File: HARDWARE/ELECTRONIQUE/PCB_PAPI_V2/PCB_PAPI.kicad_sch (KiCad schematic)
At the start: 0 parts

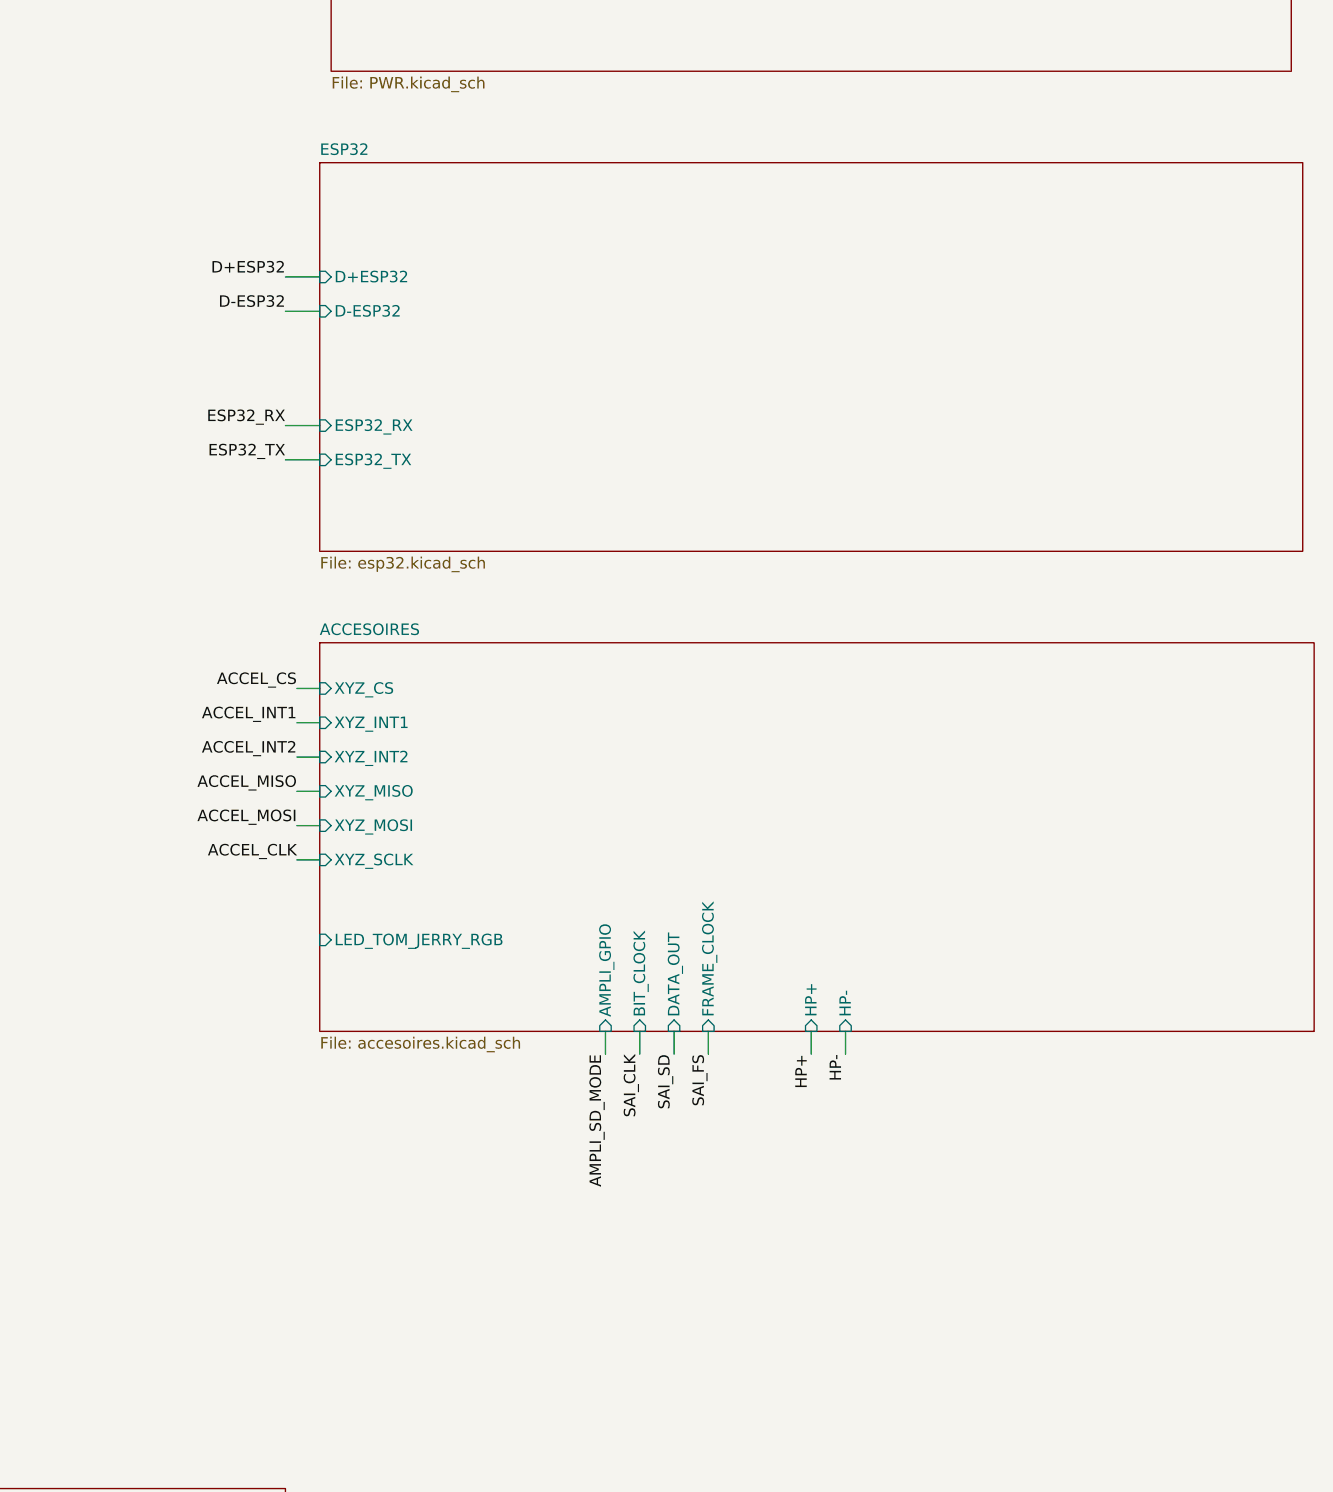
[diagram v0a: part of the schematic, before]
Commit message: up
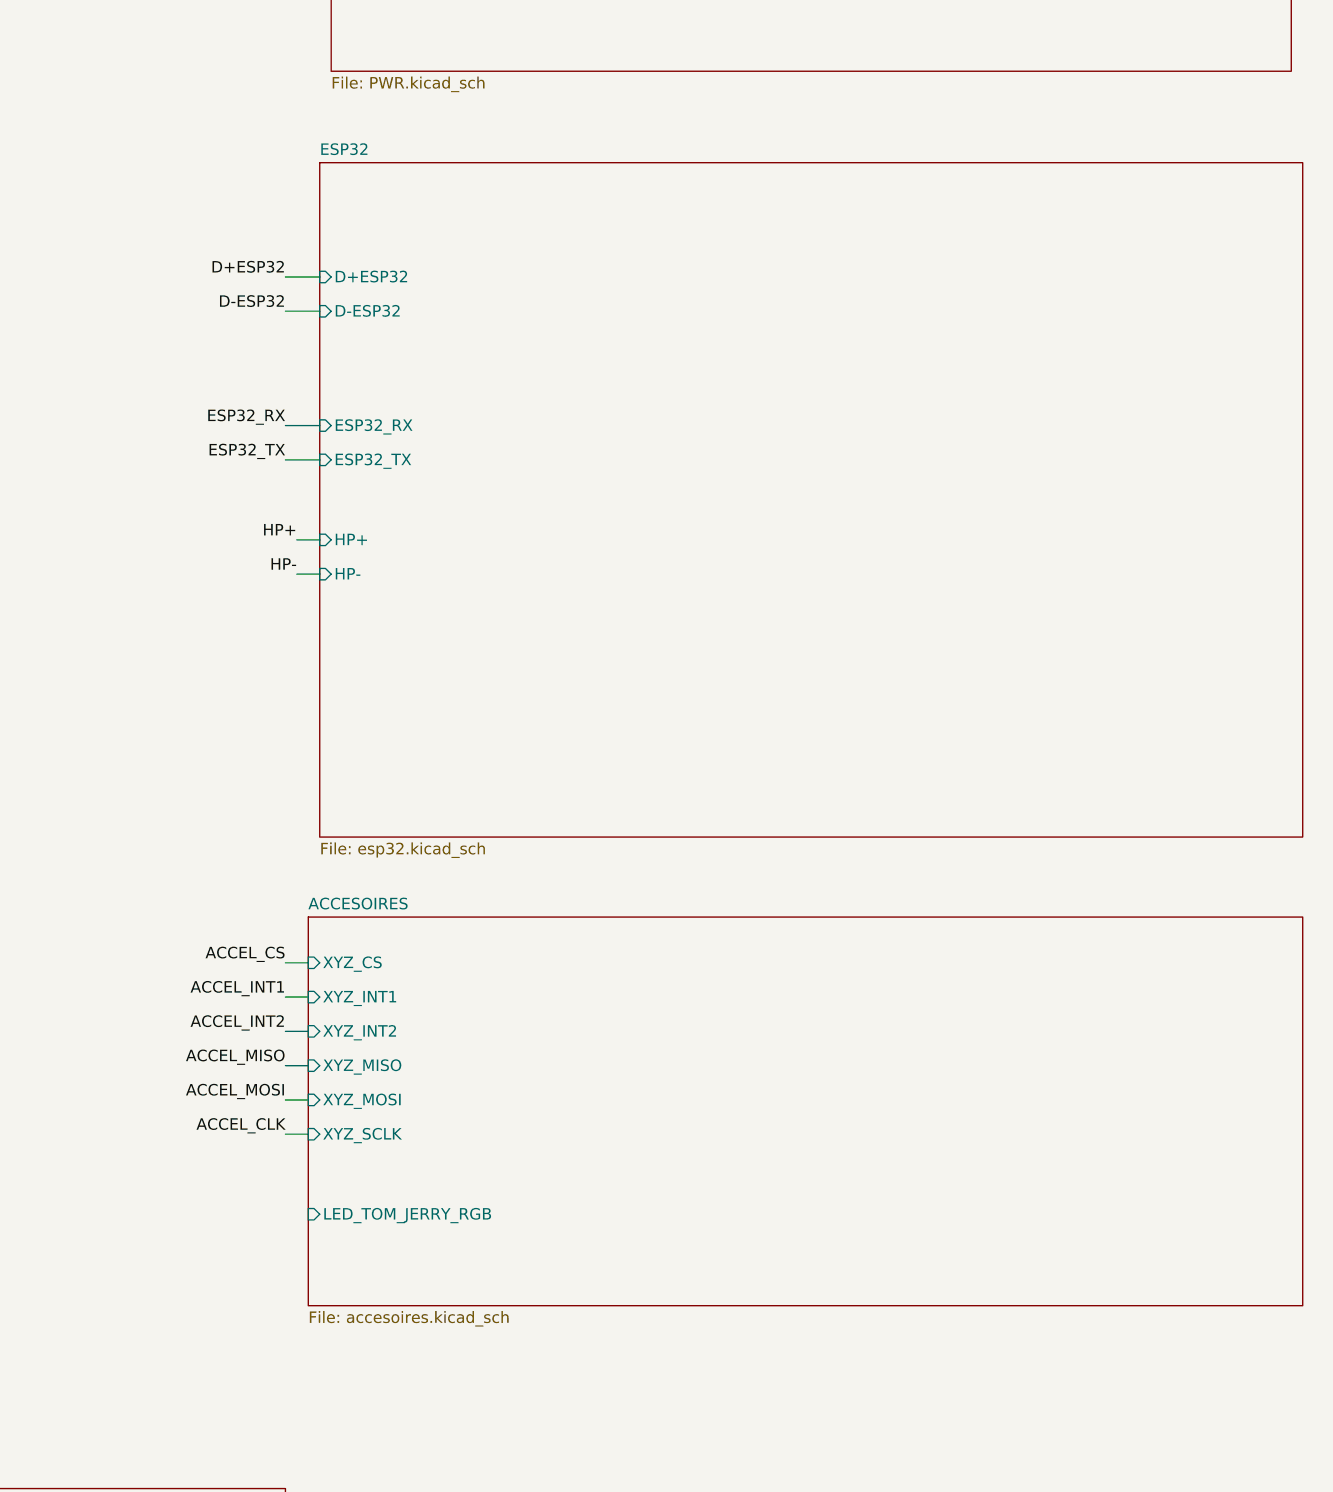
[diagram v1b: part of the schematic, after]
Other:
- sheet ACCESOIRES ports: added none; removed AMPLI_GPIO, BIT_CLOCK, DATA_OUT, FRAME_CLOCK, HP+, HP-
- sheet ESP32 ports: added HP+, HP-; removed none
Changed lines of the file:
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@@
-	(wire
-		(pts
-			(xy 496.57 204.47) (xy 496.57 201.93)
-		)
-		(stroke
-			(width 0)
-			(type default)
-		)
-	)
 	(wire
 		(pts
@@
 	(wire
 		(pts
-			(xy 435.61 167.64) (xy 438.15 167.64)
+			(xy 434.34 198.12) (xy 436.88 198.12)
 		)
 		(stroke
@@
 	(wire
 		(pts
-			(xy 435.61 163.83) (xy 438.15 163.83)
+			(xy 434.34 194.31) (xy 436.88 194.31)
 		)
 		(stroke
@@
 	(wire
 		(pts
-			(xy 435.61 175.26) (xy 438.15 175.26)
+			(xy 434.34 205.74) (xy 436.88 205.74)
 		)
 		(stroke
@@
 	(wire
 		(pts
-			(xy 435.61 179.07) (xy 438.15 179.07)
+			(xy 434.34 209.55) (xy 436.88 209.55)
 		)
 		(stroke
@@
 	(wire
 		(pts
-			(xy 435.61 171.45) (xy 438.15 171.45)
+			(xy 434.34 201.93) (xy 436.88 201.93)
 		)
 		(stroke
@@
 	(wire
 		(pts
-			(xy 469.9 204.47) (xy 469.9 201.93)
-		)
-		(stroke
-			(width 0)
-			(type default)
-		)
-	)
-	(wire
-		(pts
 			(xy 278.13 248.92) (xy 278.13 252.73)
 		)
@@
 	(wire
 		(pts
+			(xy 435.61 147.32) (xy 438.15 147.32)
+		)
+		(stroke
+			(width 0)
+			(type default)
+		)
+	)
+	(wire
+		(pts
 			(xy 142.24 124.46) (xy 138.43 124.46)
 		)
@@
 	(wire
 		(pts
-			(xy 473.71 204.47) (xy 473.71 201.93)
-		)
-		(stroke
-			(width 0)
-			(type default)
-		)
-	)
-	(wire
-		(pts
 			(xy 434.34 134.62) (xy 438.15 134.62)
 		)
@@
 	(wire
 		(pts
-			(xy 477.52 204.47) (xy 477.52 201.93)
-		)
-		(stroke
-			(width 0)
-			(type default)
-		)
-	)
-	(wire
-		(pts
 			(xy 438.15 303.53) (xy 434.34 303.53)
 		)
@@
 	(wire
 		(pts
-			(xy 435.61 182.88) (xy 438.15 182.88)
-		)
-		(stroke
-			(width 0)
-			(type default)
-		)
-	)
-	(wire
-		(pts
-			(xy 481.33 204.47) (xy 481.33 201.93)
+			(xy 434.34 213.36) (xy 436.88 213.36)
 		)
 		(stroke
@@
 	(wire
 		(pts
-			(xy 492.76 204.47) (xy 492.76 201.93)
-		)
-		(stroke
-			(width 0)
-			(type default)
-		)
-	)
-	(wire
-		(pts
 			(xy 434.34 121.92) (xy 438.15 121.92)
 		)
@@
 		(pts
 			(xy 142.24 140.97) (xy 138.43 140.97)
+		)
+		(stroke
+			(width 0)
+			(type default)
+		)
+	)
+	(wire
+		(pts
+			(xy 435.61 151.13) (xy 438.15 151.13)
 		)
 		(stroke
@@
 	)
 	(label "ACCEL_INT2"
-		(at 435.61 171.45 180)
+		(at 434.34 201.93 180)
 		(effects
 			(font
@@
 	)
 	(label "ACCEL_INT1"
-		(at 435.61 167.64 180)
+		(at 434.34 198.12 180)
 		(effects
 			(font
@@
 		)
 	)
-	(label "AMPLI_SD_MODE"
-		(at 469.9 204.47 270)
-		(effects
-			(font
-				(size 1.27 1.27)
-			)
-			(justify right bottom)
-		)
-	)
 	(label "GND_CONTROLLED"
 		(at 435.61 83.82 180)
@@
 		)
 	)
-	(label "SAI_FS"
-		(at 481.33 204.47 270)
-		(effects
-			(font
-				(size 1.27 1.27)
-			)
-			(justify right bottom)
-		)
-	)
 	(label "RX_MOT1"
 		(at 182.88 248.92 90)
@@
 		)
 	)
+	(label "HP+"
+		(at 435.61 147.32 180)
+		(effects
+			(font
+				(size 1.27 1.27)
+			)
+			(justify right bottom)
+		)
+	)
 	(label "SCL_OLED"
 		(at 140.97 165.1 0)
@@
 	)
 	(label "ACCEL_CS"
-		(at 435.61 163.83 180)
+		(at 434.34 194.31 180)
 		(effects
 			(font
@@
 		)
 	)
-	(label "HP+"
-		(at 492.76 204.47 270)
-		(effects
-			(font
-				(size 1.27 1.27)
-			)
-			(justify right bottom)
-		)
-	)
 	(label "GPIO_MOT2"
 		(at 142.24 115.57 0)
@@
 		)
 	)
-	(label "SAI_CLK"
-		(at 473.71 204.47 270)
-		(effects
-			(font
-				(size 1.27 1.27)
-			)
-			(justify right bottom)
-		)
-	)
 	(label "SWCLK"
 		(at 57.15 31.75 90)
@@
 		)
 	)
-	(label "HP-"
-		(at 496.57 204.47 270)
-		(effects
-			(font
-				(size 1.27 1.27)
-			)
-			(justify right bottom)
-		)
-	)
 	(label "GPIO_MOT2"
 		(at 199.39 248.92 90)
@@
 	)
 	(label "ACCEL_MOSI"
-		(at 435.61 179.07 180)
+		(at 434.34 209.55 180)
 		(effects
 			(font
@@
 	)
 	(label "ACCEL_CLK"
-		(at 435.61 182.88 180)
+		(at 434.34 213.36 180)
 		(effects
 			(font
@@
 		)
 	)
-	(label "SAI_SD"
-		(at 477.52 204.47 270)
-		(effects
-			(font
-				(size 1.27 1.27)
-			)
-			(justify right bottom)
-		)
-	)
 	(label "TX_MOT1"
 		(at 140.97 97.79 0)
@@
 	)
 	(label "ACCEL_MISO"
-		(at 435.61 175.26 180)
+		(at 434.34 205.74 180)
 		(effects
 			(font
@@
 			)
 			(justify left bottom)
+		)
+	)
+	(label "HP-"
+		(at 435.61 151.13 180)
+		(effects
+			(font
+				(size 1.27 1.27)
+			)
+			(justify right bottom)
 		)
 	)
@@
 	)
 	(sheet
-		(at 438.15 158.75)
+		(at 436.88 189.23)
 		(size 110.49 43.18)
 		(exclude_from_sim no)
@@
 		)
 		(property "Sheetname" "ACCESOIRES"
-			(at 438.15 158.0384 0)
+			(at 436.88 188.5184 0)
 			(effects
 				(font
@@
 		)
 		(property "Sheetfile" "accesoires.kicad_sch"
-			(at 438.15 202.5146 0)
+			(at 436.88 232.9946 0)
 			(effects
 				(font
@@
 			)
 		)
-		(pin "AMPLI_GPIO" input
-			(at 469.9 201.93 270)
+		(pin "XYZ_CS" input
+			(at 436.88 194.31 180)
 			(effects
 				(font
@@
 			)
 		)
-		(pin "BIT_CLOCK" input
-			(at 473.71 201.93 270)
+		(pin "XYZ_INT1" input
+			(at 436.88 198.12 180)
 			(effects
 				(font
@@
 			)
 		)
-		(pin "DATA_OUT" input
-			(at 477.52 201.93 270)
+		(pin "XYZ_INT2" input
+			(at 436.88 201.93 180)
 			(effects
 				(font
@@
 			)
 		)
-		(pin "FRAME_CLOCK" input
-			(at 481.33 201.93 270)
+		(pin "XYZ_MISO" input
+			(at 436.88 205.74 180)
 			(effects
 				(font
@@
 			)
 		)
-		(pin "HP+" input
-			(at 492.76 201.93 270)
+		(pin "XYZ_MOSI" input
+			(at 436.88 209.55 180)
 			(effects
 				(font
@@
 			)
 		)
-		(pin "HP-" input
-			(at 496.57 201.93 270)
+		(pin "XYZ_SCLK" input
+			(at 436.88 213.36 180)
 			(effects
 				(font
@@
 			)
 		)
-		(pin "XYZ_CS" input
-			(at 438.15 163.83 180)
-			(effects
-				(font
-					(size 1.27 1.27)
-				)
-				(justify left)
-			)
-		)
-		(pin "XYZ_INT1" input
-			(at 438.15 167.64 180)
-			(effects
-				(font
-					(size 1.27 1.27)
-				)
-				(justify left)
-			)
-		)
-		(pin "XYZ_INT2" input
-			(at 438.15 171.45 180)
-			(effects
-				(font
-					(size 1.27 1.27)
-				)
-				(justify left)
-			)
-		)
-		(pin "XYZ_MISO" input
-			(at 438.15 175.26 180)
-			(effects
-				(font
-					(size 1.27 1.27)
-				)
-				(justify left)
-			)
-		)
-		(pin "XYZ_MOSI" input
-			(at 438.15 179.07 180)
-			(effects
-				(font
-					(size 1.27 1.27)
-				)
-				(justify left)
-			)
-		)
-		(pin "XYZ_SCLK" input
-			(at 438.15 182.88 180)
-			(effects
-				(font
-					(size 1.27 1.27)
-				)
-				(justify left)
-			)
-		)
 		(pin "LED_TOM_JERRY_RGB" input
-			(at 438.15 191.77 180)
+			(at 436.88 222.25 180)
 			(effects
 				(font
@@
 	(sheet
 		(at 438.15 105.41)
-		(size 109.22 43.18)
+		(size 109.22 74.93)
 		(exclude_from_sim no)
 		(in_bom yes)
@@
 		)
 		(property "Sheetfile" "esp32.kicad_sch"
-			(at 438.15 149.1746 0)
+			(at 438.15 180.9246 0)
 			(effects
 				(font
@@
 			(effects
 				(font
+					(size 1.27 1.27)
+				)
+				(justify left)
+			)
+		)
+		(pin "HP+" input
+			(at 438.15 147.32 180)
+			(effects
+				(font
+					(size 1.27 1.27)
+				)
+				(justify left)
+			)
+		)
+		(pin "HP-" input
+			(at 438.15 151.13 180)
+			(effects
+				(font
